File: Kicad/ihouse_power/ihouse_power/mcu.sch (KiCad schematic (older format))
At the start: 108 parts, among them J13 RJ33_Shielded, J20 Conn_02x05_Top_Bottom, J3 Conn_01x20, J4 Conn_01x20, M1 stm32f1_module, Q1 IRF7403, Q2 IRF7403, Q3 IRF7403, Q4 IRF7403, Q5 BC847, U10 MAX232, U11 L7805, U6 EL814, U7 EL814, U8 EL814, U9 24LC32

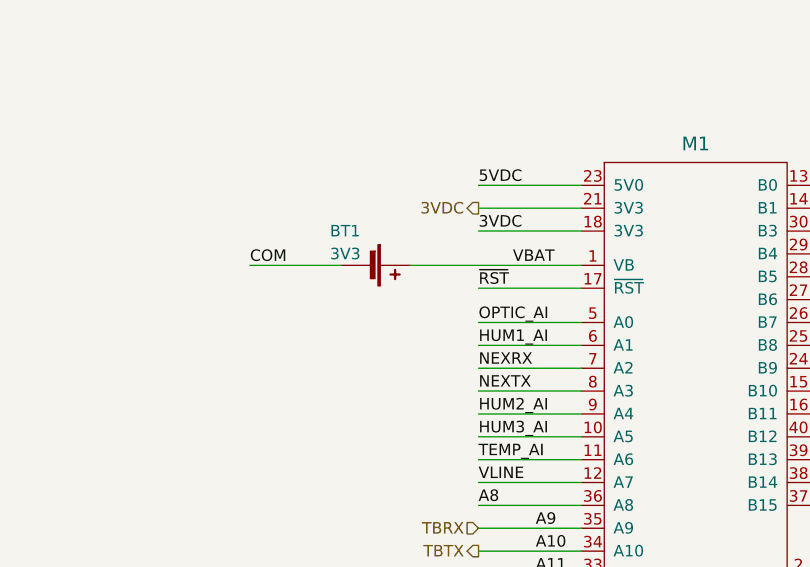
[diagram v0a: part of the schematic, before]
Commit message: 20190517
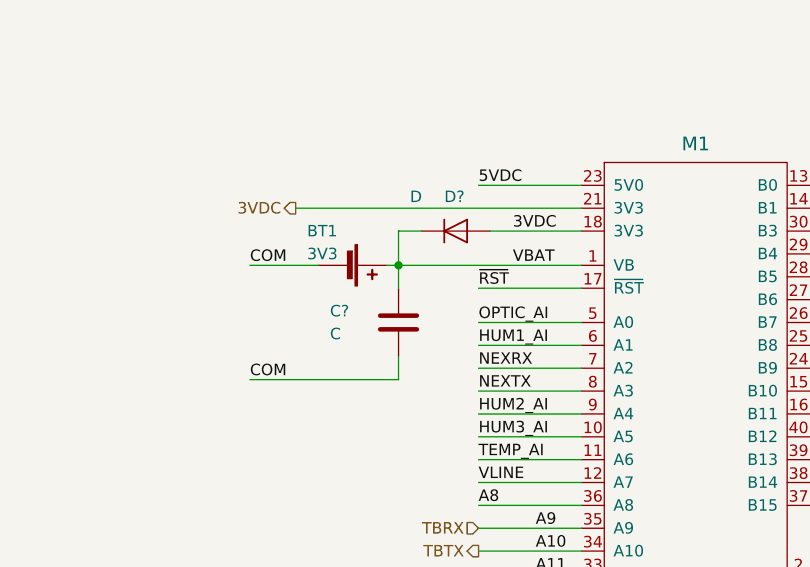
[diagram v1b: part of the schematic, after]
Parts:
- added C?: C, Capacitor_SMD:C_0805_2012Metric_Pad1.15x1.40mm_HandSolder, symbol Device:C
- added D?: D, Diode_SMD:D_MiniMELF, symbol Device:D
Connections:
- net 3VDC: now also D?.2 (A)
- net COM1: now also C?.2
- net VBAT: now also C?.1, D?.1 (K)
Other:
- moved on the sheet: BT1
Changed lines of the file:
@@
 L Device:Battery_Cell BT1
 U 1 1 5CD63D8E
-P 6150 4600
-F 0 "BT1" V 6000 4450 50  0000 L CNN
-F 1 "3V3" V 6100 4450 50  0000 L CNN
-F 2 "1220 Battery Holder:Battery_holder_1220" V 6150 4660 50  0001 C CNN
-F 3 "~" V 6150 4660 50  0001 C CNN
-	1    6150 4600
-	0    1    1    0
-$EndComp
-Wire Wire Line
-	7100 4600 6350 4600
+P 6050 4600
+F 0 "BT1" V 5900 4450 50  0000 L CNN
+F 1 "3V3" V 6000 4450 50  0000 L CNN
+F 2 "1220 Battery Holder:Battery_holder_1220" V 6050 4660 50  0001 C CNN
+F 3 "~" V 6050 4660 50  0001 C CNN
+	1    6050 4600
+	0    1    1    0
+$EndComp
 $Comp
 L Memory_EEPROM:24LC32 U9
@@
 	0    1    1    0
 $EndComp
-Wire Wire Line
-	7100 4350 6650 4350
 $Comp
 L Device:CP C11
@@
 Text HLabel 8500 5650 2    50   Output ~ 0
 ~TBCMD
-Wire Wire Line
-	7100 4450 6650 4450
 Wire Wire Line
 	7100 4850 6650 4850
@@
 Text Label 11350 4600 0    50   ~ 0
 3VDC
-Text Label 6650 4450 0    50   ~ 0
+Text Label 6800 4450 0    50   ~ 0
 3VDC
 Text Label 8350 5350 2    50   ~ 0
@@
 QCH_D3
 Wire Wire Line
-	5650 4600 6050 4600
+	5650 4600 5950 4600
 Text Label 3100 7700 2    50   ~ 0
 OPTIC_AI
@@
 Wire Wire Line
 	4250 2350 4350 2350
-Text HLabel 6650 4350 0    50   Output ~ 0
-3VDC
 $Comp
 L Connector:RJ33_Shielded J13
@@
 Text Notes 10300 9200 0    50   ~ 0
 PWM1 - WC duru pasvietimas\nPWM2 - vonios duru pasvietimas
+Text HLabel 5850 4350 0    50   Output ~ 0
+3VDC
+Wire Wire Line
+	7100 4600 6300 4600
+Wire Wire Line
+	6400 4450 6300 4450
+Wire Wire Line
+	6300 4450 6300 4600
+Connection ~ 6300 4600
+Wire Wire Line
+	6300 4600 6250 4600
+Wire Wire Line
+	5850 4350 7100 4350
+Wire Wire Line
+	7100 4450 6700 4450
+$Comp
+L Device:D D?
+U 1 1 5CEB3D8E
+P 6550 4450
+F 0 "D?" H 6500 4600 50  0000 L CNN
+F 1 "D" H 6350 4600 50  0000 L CNN
+F 2 "Diode_SMD:D_MiniMELF" H 6550 4450 50  0001 C CNN
+F 3 "~" H 6550 4450 50  0001 C CNN
+	1    6550 4450
+	1    0    0    -1
+$EndComp
+$Comp
+L Device:C C?
+U 1 1 5D3B6207
+P 6300 4850
+F 0 "C?" H 6000 4900 50  0000 L CNN
+F 1 "C" H 6000 4800 50  0000 L CNN
+F 2 "Capacitor_SMD:C_0805_2012Metric_Pad1.15x1.40mm_HandSolder" H 6338 4700 50  0001 C CNN
+F 3 "~" H 6300 4850 50  0001 C CNN
+	1    6300 4850
+	1    0    0    -1
+$EndComp
+Wire Wire Line
+	6300 4700 6300 4600
+Wire Wire Line
+	6300 5000 6300 5100
+Wire Wire Line
+	6300 5100 5650 5100
+Text Label 5650 5100 0    50   ~ 0
+COM
 $EndSCHEMATC
